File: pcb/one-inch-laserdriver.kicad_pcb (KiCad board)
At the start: 2 copper layers, 25.8 x 25.8 mm, 22 parts, among them J1 Conn_Coaxial, J2 Conn_Coaxial, J3 Power, U1 iC-HK, U3 HT75xx-1-SOT89

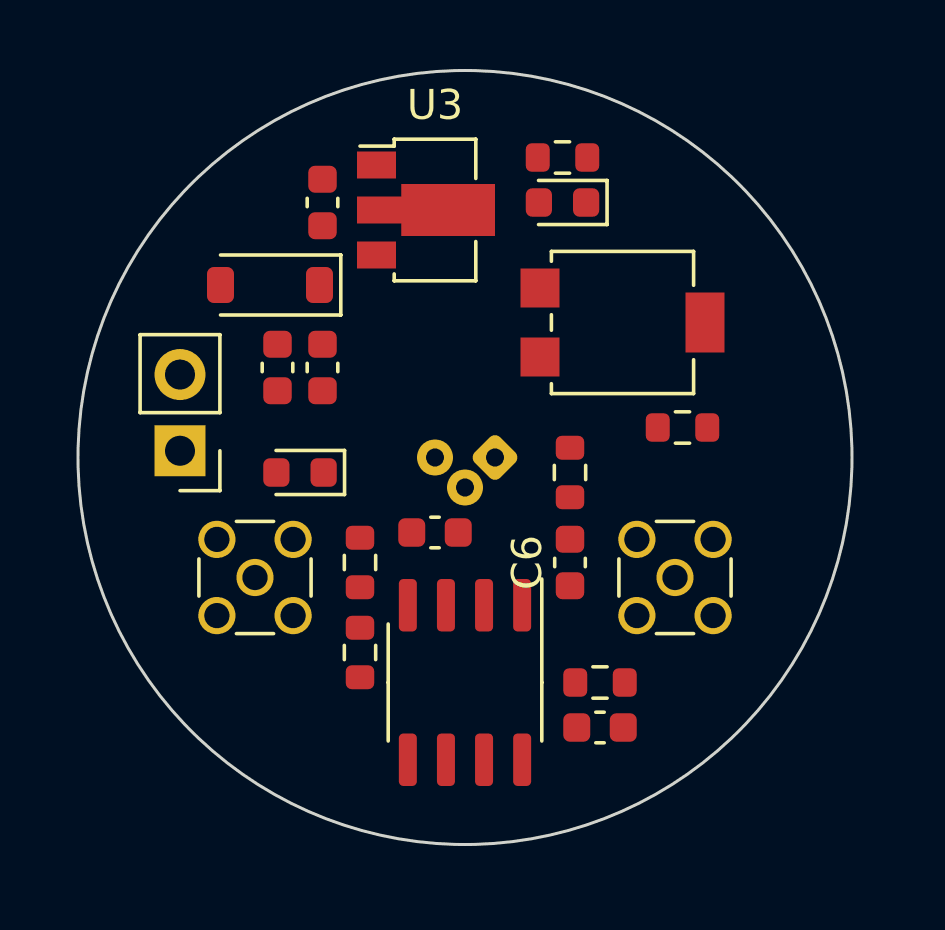
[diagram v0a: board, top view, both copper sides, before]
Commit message: ic-HKb version done
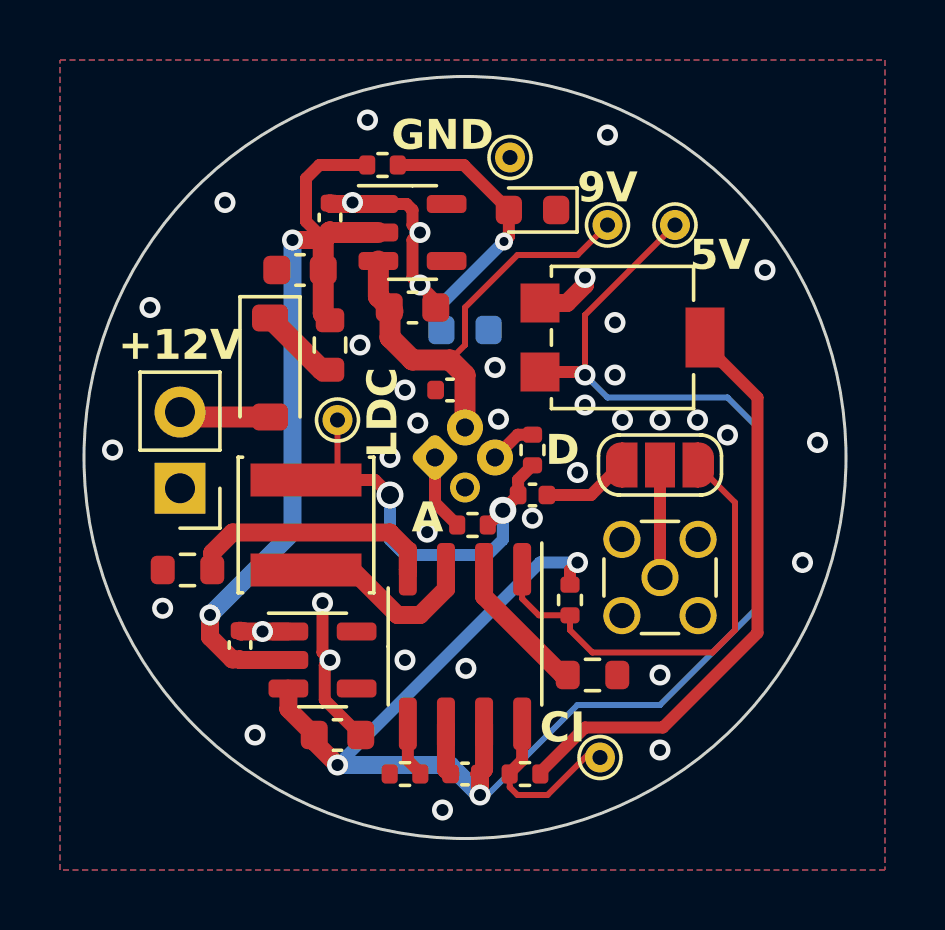
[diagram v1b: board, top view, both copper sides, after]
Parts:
- removed J1: Conn_Coaxial, Connector_Coaxial:MMCX_Molex_73415-1471_Vertical
- added C7: 0.1uF, Capacitor_SMD:C_0402_1005Metric, F.Cu at (42.5, 56.2)
- added C8: 10uF, Capacitor_SMD:C_0603_1608Metric, F.Cu at (48.2, 45.0)
- added JP1: SolderJumper_3_Bridged12, Jumper:SolderJumper-3_P1.3mm_Open_RoundedPad1.0x1.5mm_NumberLabels, F.Cu at (56.5, 50.2)
- added L1: 22uH, Inductor_SMD:L_Sunlord_SWPA4018S, F.Cu at (44.7, 52.2)
- added R7: 10, Resistor_SMD:R_0603_1608Metric, F.Cu at (45.5, 46.2)
- added R8: 10k, Resistor_SMD:R_0402_1005Metric, F.Cu at (48.0, 60.5)
- added R9: 47*, Resistor_SMD:R_0402_1005Metric, F.Cu at (52.2, 49.8)
- added TP1: 9V, TestPoint:TestPoint_THTPad_D1.0mm_Drill0.5mm, F.Cu at (54.8, 42.2)
- added TP2: 5V, TestPoint:TestPoint_THTPad_D1.0mm_Drill0.5mm, F.Cu at (57.0, 42.2)
- added TP3: GND, TestPoint:TestPoint_THTPad_D1.0mm_Drill0.5mm, F.Cu at (51.5, 40.0)
- added TP4: LDC, TestPoint:TestPoint_THTPad_D1.0mm_Drill0.5mm, F.Cu at (45.8, 48.8)
- added TP5: CI, TestPoint:TestPoint_THTPad_D1.0mm_Drill0.5mm, F.Cu at (54.5, 60.0)
- added TP6: Hole, TestPoint:TestPoint_THTPad_D1.0mm_Drill0.5mm, F.Cu at (50.0, 51.0)
- added U2: HT7590-3, Package_TO_SOT_SMD:SOT-23-5, F.Cu at (48.2, 42.5)
- C1, C4, C5, C6: footprint Capacitor_SMD:C_0603_1608Metric -> Capacitor_SMD:C_0402_1005Metric
- D2: moved to B.Cu
- R1, R5, R6: footprint Resistor_SMD:R_0603_1608Metric -> Resistor_SMD:R_0402_1005Metric
- R2, R3: value 3.3 -> 1
- R4: value 1k -> 10k; footprint Resistor_SMD:R_0603_1608Metric -> Resistor_SMD:R_0402_1005Metric
- U3: value HT75xx-1-SOT89 -> HT7550-2; footprint Package_TO_SOT_SMD:SOT-89-3 -> Package_TO_SOT_SMD:SOT-23-5
- moved C3 17.8 mm to (45.8, 59.2), turned to 0 degrees
- moved U3 15.5 mm to (45.2, 56.8)
- moved R6 12.7 mm to (52.0, 60.5)
- moved D2 7.27 mm to (50.0, 45.8)
- moved R4 7.11 mm to (53.5, 54.8)
- moved R3 6.37 mm to (40.8, 53.8), turned to 180 degrees
- moved R1 6.01 mm to (47.2, 40.2), turned to 0 degrees
- moved C1 5.01 mm to (45.5, 42.0), turned to 90 degrees
- moved C5 4.78 mm to (49.5, 47.8)
- moved C4 4.76 mm to (50.0, 60.5), turned to 180 degrees
- moved R5 3.69 mm to (50.2, 52.2), turned to 180 degrees
- moved C2 3.34 mm to (44.5, 43.8), turned to 180 degrees
- moved D4 2.75 mm to (43.5, 47.0), turned to -90 degrees
- moved C6 2.57 mm to (52.2, 51.2), turned to 180 degrees
- moved LD1 2.00 mm to (49.0, 50.0), turned to 0 degrees
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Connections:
- C1 pad 1: Net-(D4-K) -> Net-(U2-VIN)
- C2 pad 1: Net-(D4-K) -> Net-(U2-VIN)
- C5 pad 1: +5V -> +9V
- C6 pad 1: Net-(J2-In) -> Net-(JP1-A)
- D2 pad 2: Net-(D2-A) -> Net-(D1-A)
- LD1 pad 2: +5V -> +9V
- LD1 pad 3: unconnected-(LD1-Pad3) -> Net-(LD1-Pad3)
- R1 pad 1: +5V -> Net-(U2-VIN)
- R4 pad 2: Net-(D2-A) -> +5V
- U1 pad 5: unconnected-(U1-EN2-Pad5) -> Net-(U1-EN2)
- U3 pad 2: Net-(D4-K) -> Net-(U2-VIN)
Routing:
- net +5V: track 0.00 -> 54.6 mm, vias 0 -> 4
- net Net-(U2-VIN): track 0.00 -> 27.6 mm, vias 0 -> 2
- net Net-(R6-Pad2): track 0.00 -> 19.8 mm
- net GND: track 0.00 -> 17.1 mm, vias 0 -> 38
- net Net-(JP1-B): track 0.00 -> 15.7 mm
- net +9V: track 0.00 -> 15.5 mm
- net Net-(C6-Pad2): track 0.00 -> 15.3 mm, vias 0 -> 2
- net Net-(D1-A): track 0.00 -> 9.26 mm, vias 0 -> 1
- net Net-(U1-AGND2): track 0.00 -> 8.43 mm
- net Net-(U1-LDK): track 0.00 -> 6.30 mm
- net Net-(U1-CI): track 0.00 -> 6.28 mm
- net Net-(U1-AGND1): track 0.00 -> 4.78 mm
- net Net-(J2-In): track 0.00 -> 3.75 mm
- net Net-(D4-A): track 0.00 -> 3.07 mm
- net Net-(JP1-A): track 0.00 -> 2.88 mm
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- added copper zone on B.Cu, net GND
- added copper zone on F.Cu, net GND
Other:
- board size 25.8 x 25.8 mm -> 25.4 x 25.4 mm
- board text added: "+12V"
- board text added: "/One-Inch-LaserDriver"
- board text added: "2023"
- board text added: "LDA"
- board text added: "Mitch Cox"
- board text added: "github.com/WitsOCLab"
